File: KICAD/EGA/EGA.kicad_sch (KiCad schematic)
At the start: 32 parts, among them J1 12V, J2 PWM MOTOR, J3 LCD 20x4, J4 RTC, J5 MEMORY SD, J6 HC-SR04, M1 Fan_3pin, Q1 IRLZ44N, Q2 IRLZ44N, SW1 RESET, U1 LM7805_TO220, U2 LM317_TO-220, U3 Pico

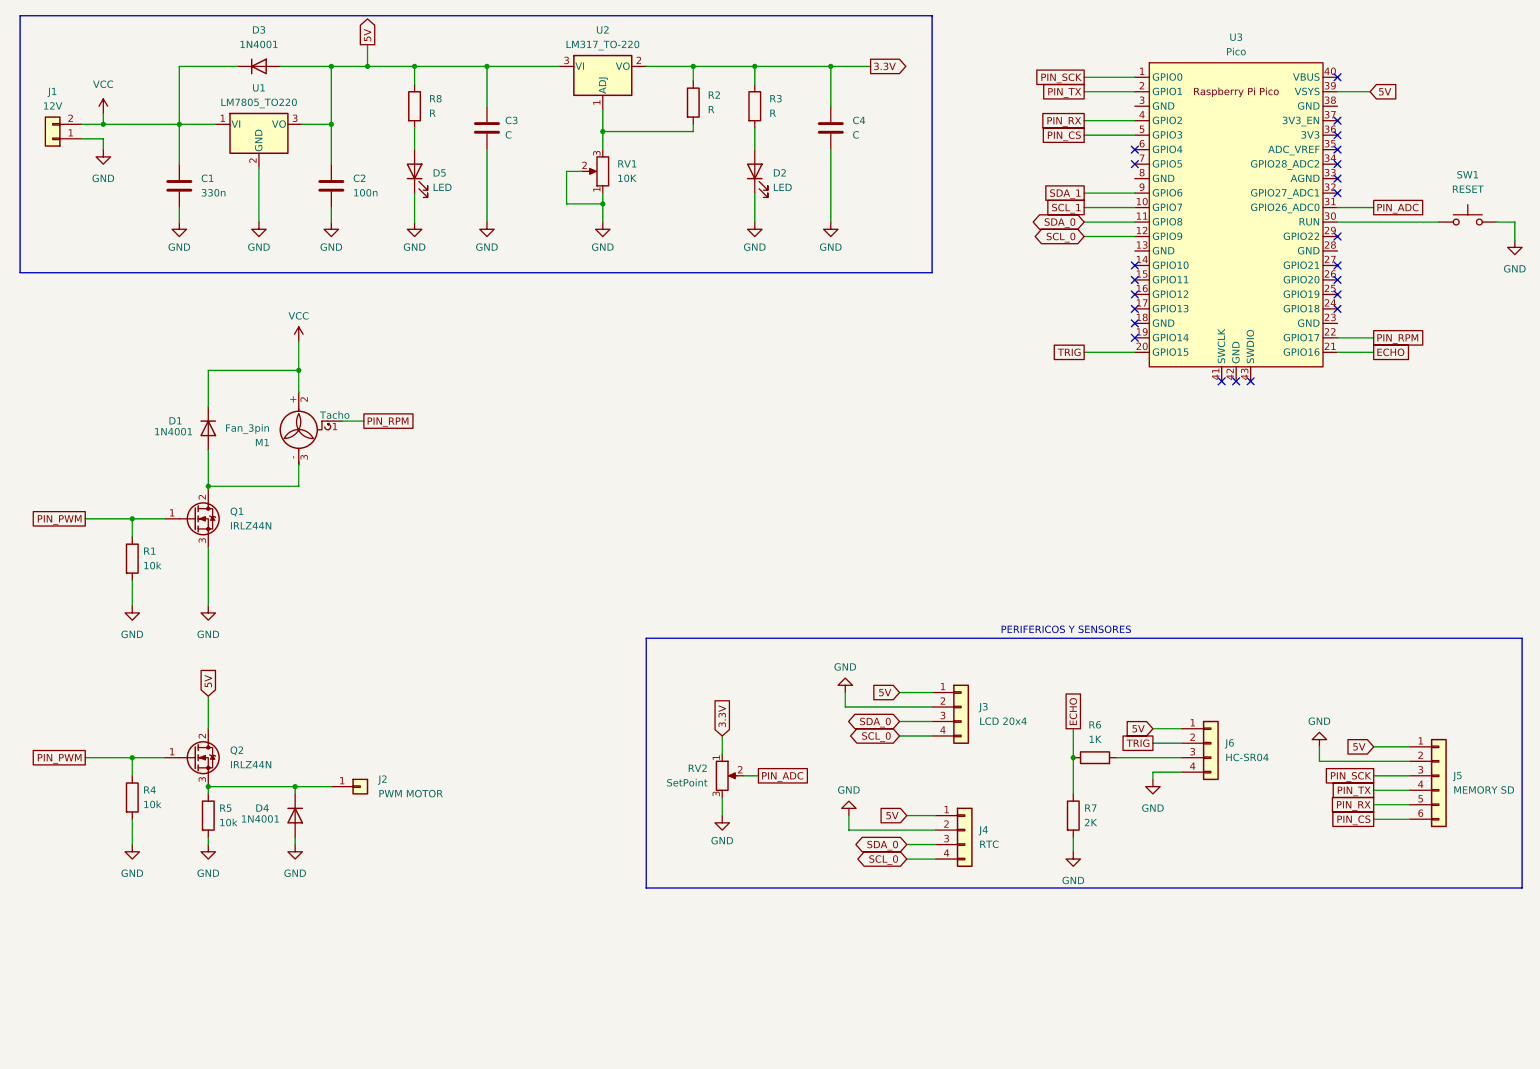
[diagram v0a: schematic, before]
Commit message: Actualizacion KICAD 13/7/2025
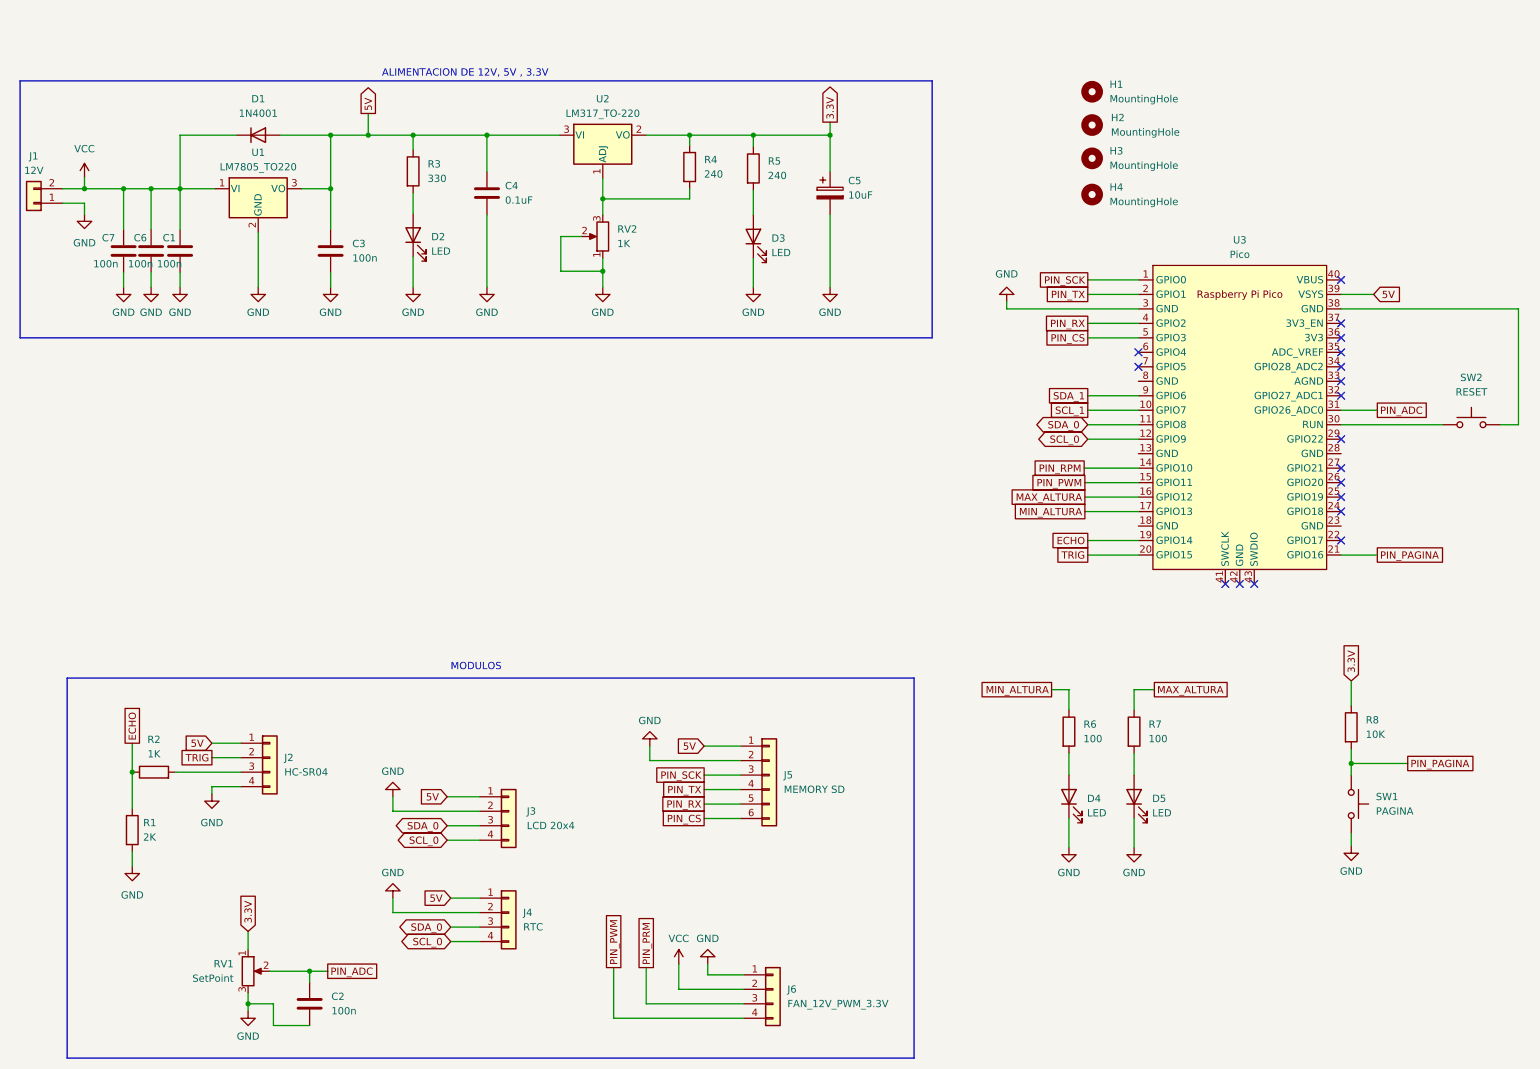
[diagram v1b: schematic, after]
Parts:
- removed D1, D4: 1N4001, Diode_THT:D_DO-41_SOD81_P10.16mm_Horizontal, symbol Diode:1N4001
- removed J2: PWM MOTOR, symbol Connector_Generic:Conn_01x01
- removed M1: Fan_3pin, symbol Motor:Fan_3pin
- removed Q1, Q2: IRLZ44N, Package_TO_SOT_THT:TO-220-3_Vertical, symbol Transistor_FET:IRLZ44N
- removed R1, R4, R5: 10k, symbol Device:R
- added C2, C6, C7: 100n, Capacitor_THT:C_Disc_D5.0mm_W2.5mm_P2.50mm, symbol Device:C
- added D4, D5: LED, LED_THT:LED_D5.0mm, symbol Device:LED
- added H1, H2, H3, H4: MountingHole, MountingHole:MountingHole_2.1mm, symbol Mechanical:MountingHole
- added J6: FAN_12V_PWM_3.3V, Connector_PinHeader_2.00mm:PinHeader_1x04_P2.00mm_Vertical, symbol Connector_Generic:Conn_01x04
- added R6, R7: 100, Resistor_THT:R_Axial_DIN0204_L3.6mm_D1.6mm_P7.62mm_Horizontal, symbol Device:R
- added R8: 10K, Resistor_THT:R_Axial_DIN0204_L3.6mm_D1.6mm_P7.62mm_Horizontal, symbol Device:R
- added SW1: PAGINA, Button_Switch_THT:SW_PUSH_6mm_H4.3mm, symbol Switch:SW_Push
- C1: value 330n -> 100n; footprint Capacitor_THT:C_Disc_D7.5mm_W4.4mm_P5.00mm -> Capacitor_THT:C_Disc_D5.0mm_W2.5mm_P2.50mm
- C4: renamed from C3; value C -> 0.1uF; footprint (none) -> Capacitor_THT:C_Disc_D5.0mm_W2.5mm_P2.50mm
- C5: renamed from C4; value C -> 10uF; footprint (none) -> Capacitor_THT:CP_Radial_D5.0mm_P2.50mm; symbol Device:C -> Device:C_Polarized
- D2: renamed from D5; footprint (none) -> LED_THT:LED_D5.0mm
- D3: renamed from D2; footprint (none) -> LED_THT:LED_D5.0mm
- J1: footprint (none) -> Connector_Molex:Molex_KK-254_AE-6410-02A_1x02_P2.54mm_Vertical
- J2: renamed from J6; footprint (none) -> Connector_PinHeader_2.00mm:PinHeader_1x04_P2.00mm_Vertical
- J3, J4: footprint (none) -> Connector_PinHeader_2.00mm:PinHeader_1x04_P2.00mm_Vertical
- J5: footprint (none) -> Connector_PinHeader_2.00mm:PinHeader_1x06_P2.00mm_Vertical
- R1: renamed from R7; footprint (none) -> Resistor_THT:R_Axial_DIN0204_L3.6mm_D1.6mm_P7.62mm_Horizontal
- R2: renamed from R6; footprint (none) -> Resistor_THT:R_Axial_DIN0204_L3.6mm_D1.6mm_P7.62mm_Horizontal
- R3: renamed from R8; value R -> 330; footprint (none) -> Resistor_THT:R_Axial_DIN0204_L3.6mm_D1.6mm_P7.62mm_Horizontal
- R4: renamed from R2; value R -> 240; footprint (none) -> Resistor_THT:R_Axial_DIN0204_L3.6mm_D1.6mm_P7.62mm_Horizontal
- R5: renamed from R3; value R -> 240; footprint (none) -> Resistor_THT:R_Axial_DIN0204_L3.6mm_D1.6mm_P7.62mm_Horizontal
- RV1: renamed from RV2; footprint (none) -> Potentiometer_THT:Potentiometer_Vishay_T93XA_Horizontal
- RV2: renamed from RV1; value 10K -> 1K; footprint (none) -> Potentiometer_THT:Potentiometer_Vishay_T93YA_Vertical
- SW2: renamed from SW1; footprint (none) -> Button_Switch_THT:SW_PUSH_6mm_H4.3mm
- U3: footprint RPi_Pico:RPi_Pico_SMD_TH -> MCU_RaspberryPi_and_Boards:RPi_Pico_SMD_TH
- renumbered C2 to C3, D3 to D1
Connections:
- net 3.3V: now also R8.1
- net ECHO: now also U3.19 (GPIO14); no longer U3.21 (GPIO16)
- net GND: now also U3.3 (GND), C2.2, C6.2, C7.2, D4.1 (K), D5.1 (K), J6.1 (Pin_1), SW1.2; no longer SW2.2
- net PIN_ADC: now also C2.1
- net PIN_PWM: now also U3.15 (GPIO11), J6.4 (Pin_4)
- net PIN_RPM: now also U3.14 (GPIO10); no longer U3.22 (GPIO17)
- net VCC: now also C6.1, C7.1, J6.2 (Pin_2)
- net MAX_ALTURA: now reaches U3.16 (GPIO12)
- net MAX_ALTURA: now also R7.1
- net MIN_ALTURA: now reaches U3.17 (GPIO13)
- net MIN_ALTURA: now also R6.1
- net at U3.38 (GND): now also SW2.2
- new net: D4.2 (A), R6.2
- new net: D5.2 (A), R7.2
- new net PIN_PAGINA: R8.2, SW1.1, U3.21 (GPIO16)
- new net PIN_PRM: J6.3 (Pin_3)
- no-connect marks 23 -> 18
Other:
- note added: "ALIMENTACION DE 12V, 5V , 3.3V"
- note added: "MODULOS"
- note removed: "PERIFERICOS Y SENSORES"
- moved on the sheet: C3, C4, D1, D2, D3, J1, J2, J3, J4, J5, R1, R2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
